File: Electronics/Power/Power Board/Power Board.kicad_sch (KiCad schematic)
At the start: 4 parts

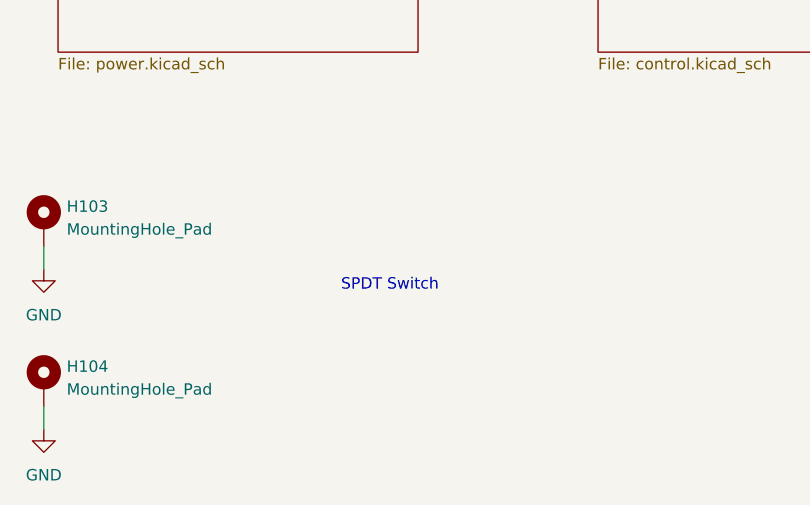
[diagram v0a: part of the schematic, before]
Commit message: Finished power board layout
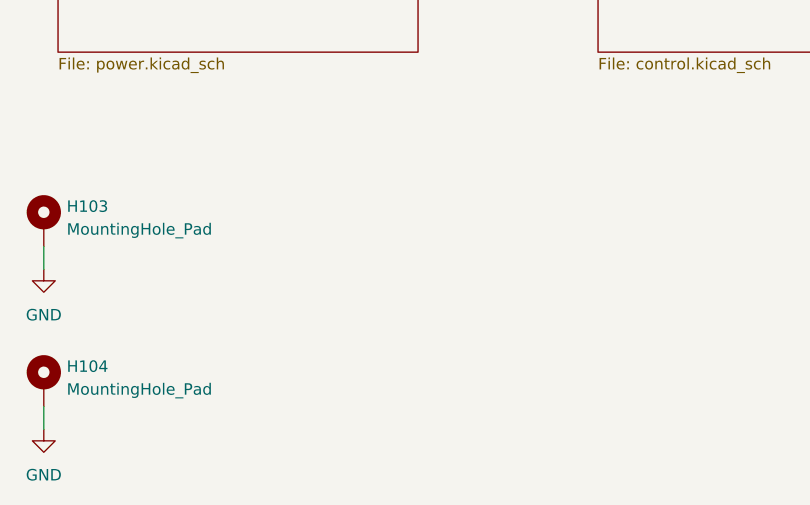
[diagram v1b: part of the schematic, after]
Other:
- note removed: "SPDT Switch"
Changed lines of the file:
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@@
     (stroke (width 0) (type default))
-  )
-  (text "SPDT Switch" (at 91.44 106.68 0)
-    (effects (font (size 1.27 1.27)) (justify left bottom))
   )
   (symbol (lib_id "power:GND") (at 34.29 121.92 0) (unit 1)
